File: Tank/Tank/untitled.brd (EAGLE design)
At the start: 94.3 x 60.9 mm, 37 parts, among them U1 L298N, U2 Atmega1284, U3 Regulator 6V, U4 Regulator 5v, X1 Led RGB, X10 Encoder Dreapta, X12 Switch power, X13 Switch reset, X14 Senzor distanta 2, X15 Senzor distanta 3, X2 Led, X3 Servo, X4 Bluetooth, X5 Senzor distanta 1, X6 Encoder Stanga, X7 Debug

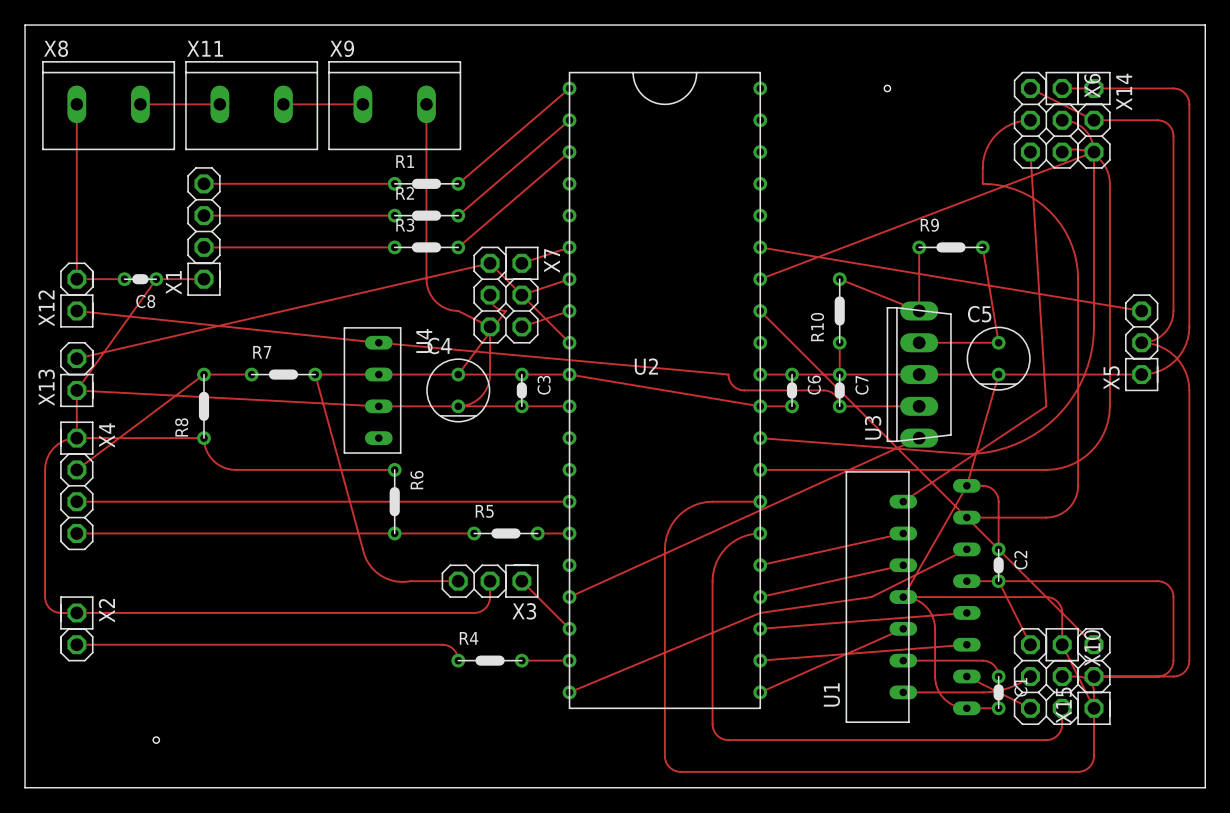
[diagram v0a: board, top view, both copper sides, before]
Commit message: laptop->pc test part
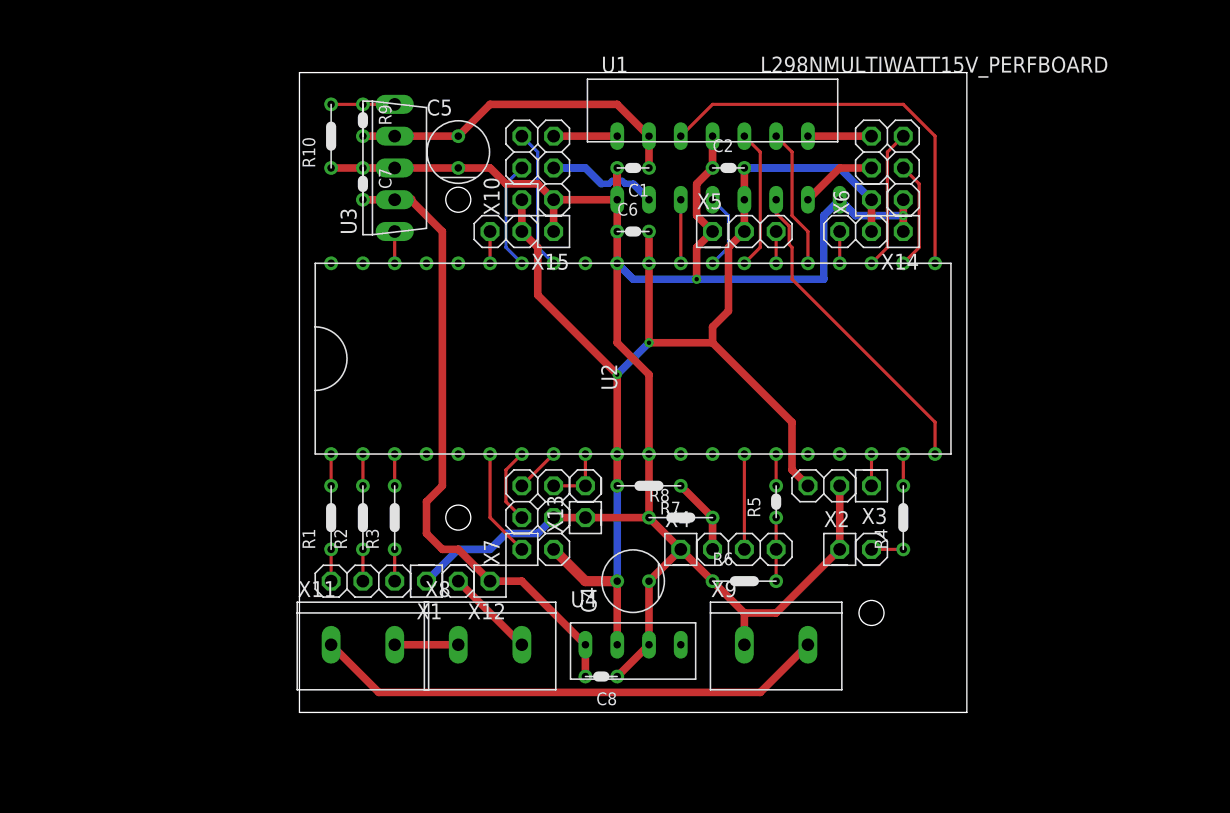
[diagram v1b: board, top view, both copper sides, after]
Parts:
- removed C3: 100nF, Passives:THT_2.54
- R5, R9: device Passives:THT_5.08 -> Passives:THT_2.54
- U1: value L298N -> L298NMULTIWATT15V_PERFBOARD; device Motors:MULTIWATT15V -> Motors:MULTIWATT15V_PERFBOARD
- X11: value (none) -> Middle battery
- X8: value (none) -> High battery
- X9: value (none) -> Low battery
- moved X2 62.6 mm to (66.0, 39.4), turned to 0 degrees
- moved X15 57.9 mm to (39.4, 64.8), turned to 180 degrees
- moved X10 57.5 mm to (40.6, 69.8), turned to 90 degrees
- moved X8 52.9 mm to (36.8, 31.8)
- moved X9 52.9 mm to (59.7, 31.8)
- moved X4 52.3 mm to (55.9, 39.4), turned to 0 degrees
- moved C1 51.1 mm to (48.3, 69.8), turned to 180 degrees
- moved C8 48.6 mm to (45.7, 29.2)
- moved R9 48.1 mm to (26.7, 73.7), turned to 270 degrees
- moved C5 46.2 mm to (34.3, 71.1)
- moved U3 45.0 mm to (29.2, 69.8)
- moved X11 44.1 mm to (26.7, 31.8)
- moved R10 43.0 mm to (24.1, 72.4)
- moved X13 41.9 mm to (44.5, 43.2)
- moved C7 41.5 mm to (26.7, 68.6)
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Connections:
- net EN_A_PWM renamed EN_D_PWM
- net EN_B_PWM renamed EN_S_PWM
- removed net B_RX: R5.1, R5.2, R6.2, U2.15, X4.4
- removed net N$37: X11.1, X8.2
- new net B_ON: R3.2, U2.3
- new net B_RX_3V3: R5.1, R6.2, X4.4
- new net B_RX_5V: R5.2, U2.15
- new net G_ON: R2.2, U2.2
- new net LED_PWM: R4.2, U2.19
- new net N$2: X11.2, X8.1
- new net R_ON: R1.2, U2.1
- new net VBATT: X12.2, X8.2
- net B: no longer R3.2, U2.3
- net D1: now also U2.26; no longer U2.35
- net D2: now also U2.24; no longer U2.34
- net D3: now also U2.35; no longer U2.33
- net EN_REG: now also U2.38; no longer U2.17
- net G: no longer R2.2, U2.2
- net GND: now also X10.4, X6.4, X7.5, X9.1; no longer C3.2, X10.1, X6.1, X7.6, X9.2
- net IN_1: now also U2.29; no longer U2.22
- net IN_2: now also U2.28; no longer U2.23
- net IN_3: now also U2.27; no longer U2.24
- net L_PWM: no longer R4.2, U2.19
- net M1_D: now also U1.2; no longer U1.3
- net M1_S: now also X6.3; no longer X6.6
- net M2_D: now also U1.3; no longer U1.2
- net M2_S: now also X6.2; no longer X6.5
- net N$43: now also X11.1, X9.2; no longer X11.2, X9.1
- net OUTA_D: now also U2.33; no longer U2.26
- net OUTA_S: now also U2.23, X6.6; no longer U2.28, X6.3
- net OUTB_D: now also U2.34; no longer U2.27
- net OUTB_S: now also U2.22, X6.5; no longer U2.29, X6.2
- net R: no longer R1.2, U2.1
- net RESET: now also X7.6; no longer X7.4
- net VCC5V: now also X10.1, X6.1, X7.4; no longer C3.1, X10.4, X6.4, X7.5
- net VIN11V: no longer X12.2, X8.1
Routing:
- net GND: track 276.5 -> 163.3 mm, vias 0 -> 2
- net VCC5V: track 169.2 -> 105.8 mm, vias 0 -> 2
- net OUTB_D: track 69.2 -> 8.67 mm
- net OUTA_S: track 52.4 -> 11.2 mm
- net OUTB_S: track 48.5 -> 8.67 mm
- net RESET: track 42.9 -> 5.08 mm
- net M2_S: track 43.9 -> 6.13 mm
- net OUTA_D: track 47.1 -> 11.2 mm
- net VIN11V: track 86.4 -> 51.0 mm
- net D3: track 37.7 -> 2.54 mm
- net N$43: track 6.35 -> 41.3 mm
- net B_RX: track 34.3 -> 0.00 mm
- net L_PWM: track 34.8 -> 2.54 mm
- net B_TX: track 39.4 -> 7.62 mm
- net M1_S: track 34.1 -> 5.08 mm
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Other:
- board size 94.3 x 60.9 mm -> 53.3 x 51.1 mm
- board text added: "DREAPTA"
- board text added: "FATA"
- board text added: "SPATE"
- board text added: "STANGA"
